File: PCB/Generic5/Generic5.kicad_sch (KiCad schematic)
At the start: 29 parts, among them J1 Conn_01x04, J2 USB-C, Q1 PMF170XP,115, U1 ESP32-PICO-MINI-02, U2 FT231XQ, U3 LMR16006+FB

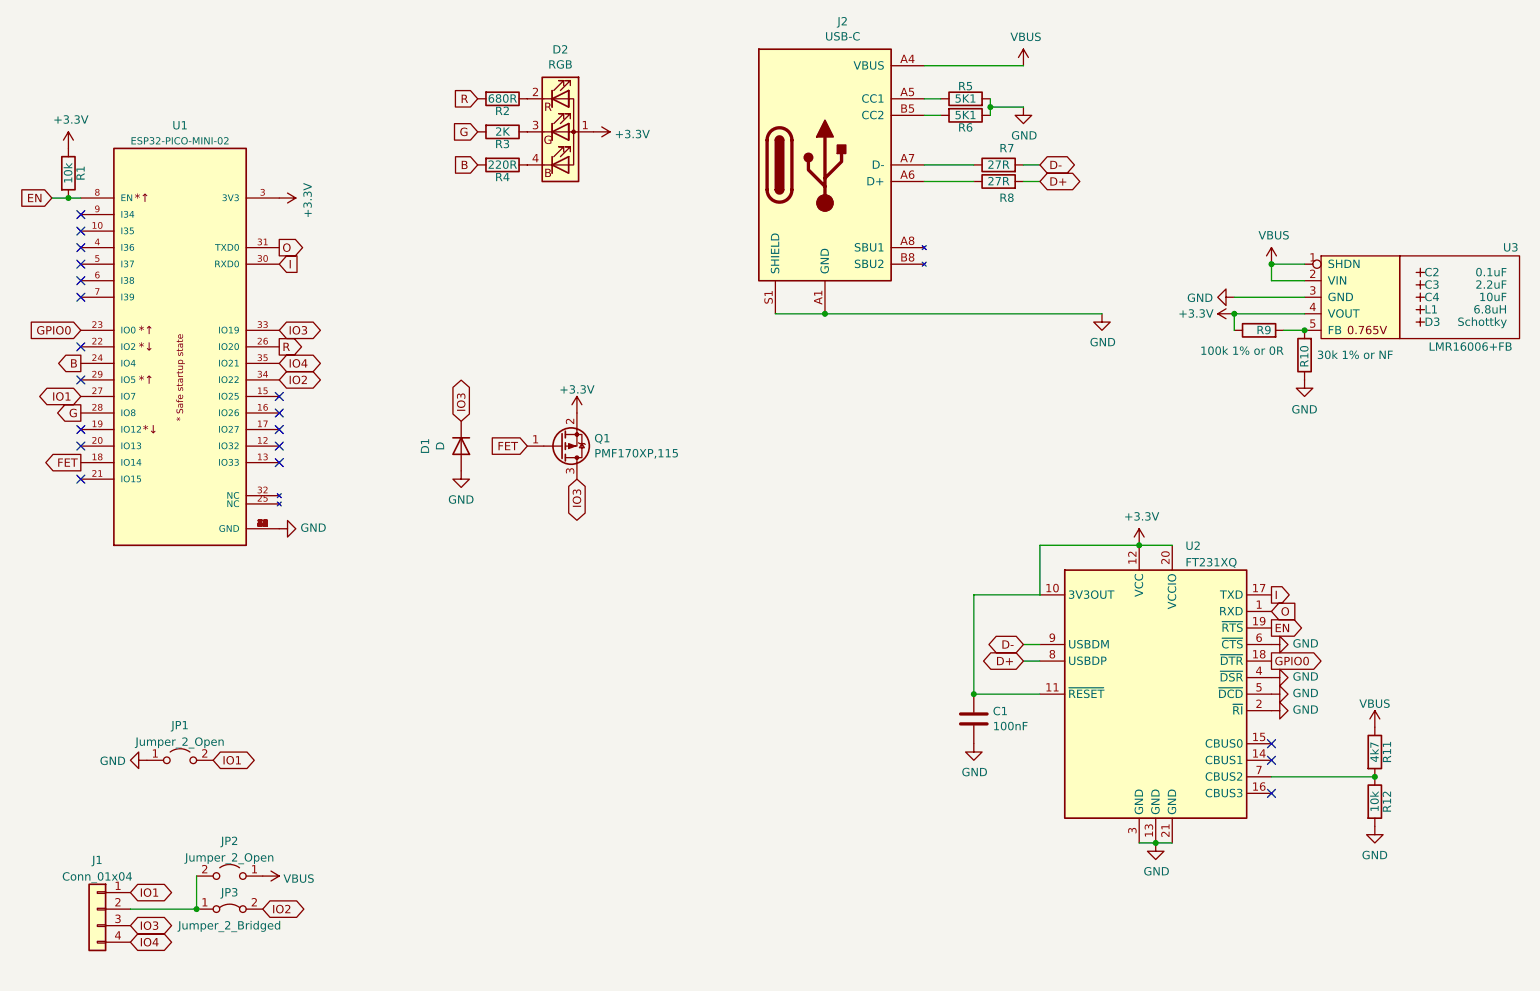
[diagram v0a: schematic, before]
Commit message: New LED Generic 5
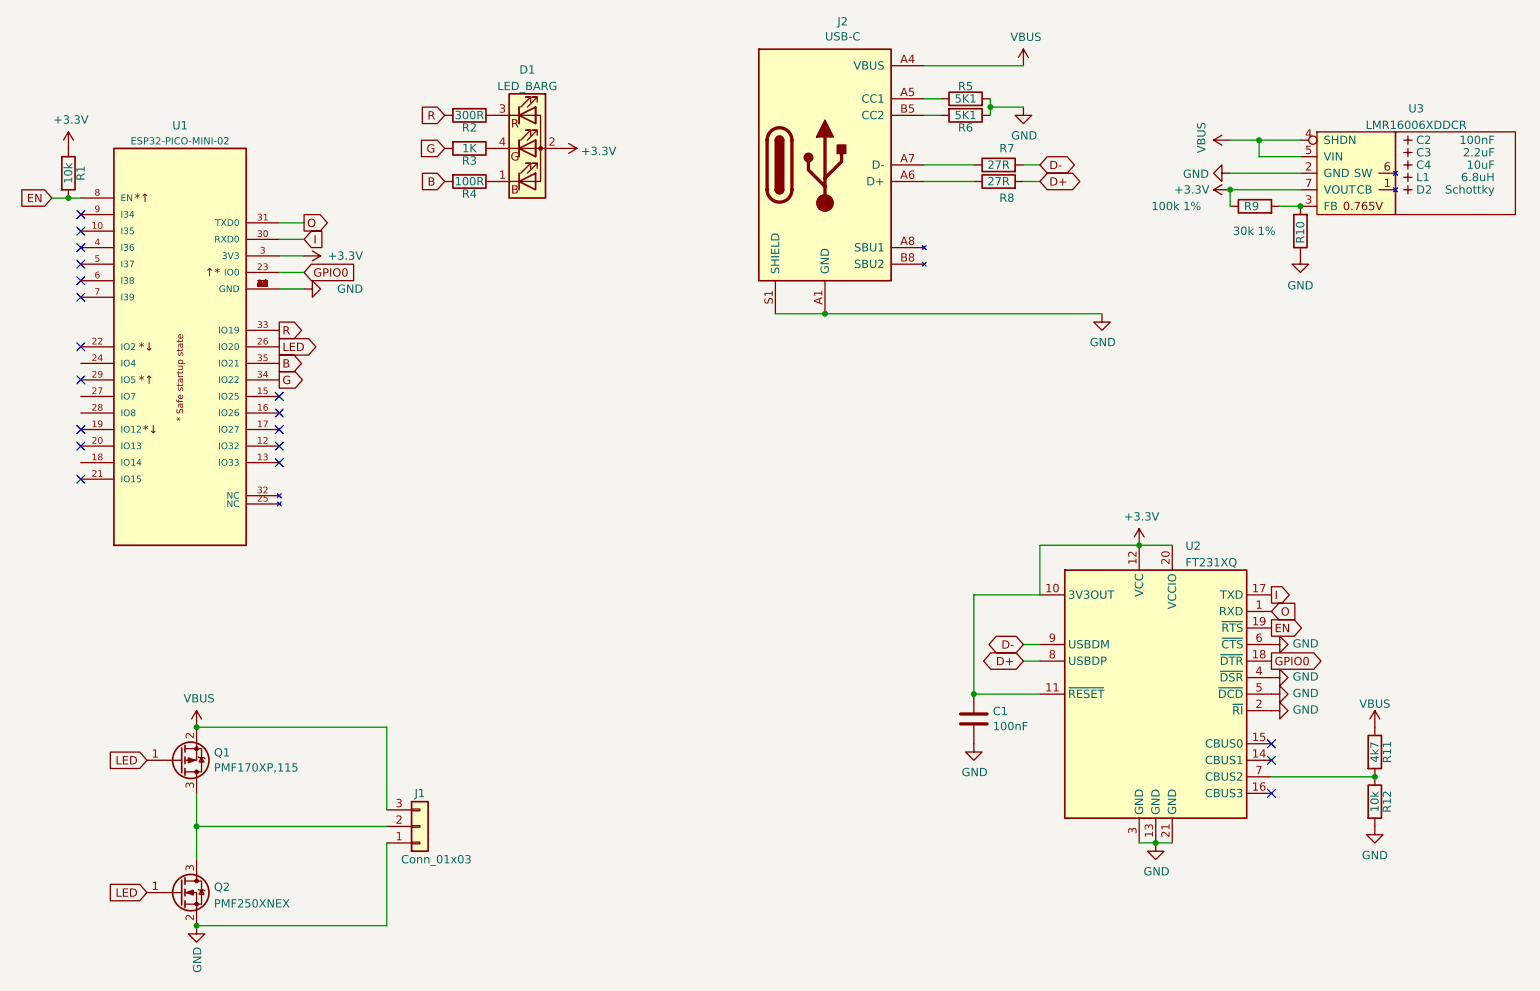
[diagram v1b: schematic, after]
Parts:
- removed D1: D, RevK:D_1206, symbol Device:D
- removed D2: RGB, RevK:LED-RGB-1.6x1.6, symbol Device:LED_ARGB
- removed D3: Schottky, RevK:Hidden, symbol RevK:Hidden
- removed J1: Conn_01x04, RevK:Molex_MiniSPOX_H4RA, symbol Connector_Generic:Conn_01x04
- removed JP1, JP2: Jumper_2_Open, RevK:Pad_0603_Open, symbol Jumper:Jumper_2_Open
- removed JP3: Jumper_2_Bridged, RevK:Pad_0603_Bridged, symbol Jumper:Jumper_2_Bridged
- removed U3: LMR16006+FB, RevK:RegulatorBlockFB, symbol RevK:LMR16006+FB
- added D1: LED_BARG, RevK:MHS190RGBCT, symbol Device:LED_BARG
- added D2: Schottky, RevK:D_1206_, symbol RevK:Hidden
- added J1: Conn_01x03, RevK:PTSM-HH-3-RA, symbol Connector_Generic:Conn_01x03
- added Q2: PMF250XNEX, RevK:SOT-323_SC-70, symbol RevK:NX7002AK
- added U3: LMR16006XDDCR, RevK:SOT-23-Thin-6-Reg, symbol RevK:LMR16006XDDCR
- C2: value 0.1uF -> 100nF; footprint RevK:Hidden -> RevK:C_0603_; LCSC Part # (none) -> C30926
- C3: footprint RevK:Hidden -> RevK:C_0805_; LCSC Part # (none) -> C19110; Note 0603 or 0805 -> (none)
- C4: footprint RevK:Hidden -> RevK:C_0805_; LCSC Part # (none) -> C17024; Note 0603 or 0805 -> (none)
- J2: footprint RevK:USC16-TR-Round -> RevK:USC16-TR-PTH
- L1: footprint RevK:Hidden -> RevK:L_4x4_; LCSC Part # (none) -> C354575; Manufacturer Laird -> (none); Part No TYA4020 -> (none)
- Q1: footprint Package_TO_SOT_SMD:SOT-323_SC-70 -> RevK:SOT-323_SC-70
- R10: value 30k 1% or NF -> 30k 1%; LCSC Part # (none) -> C100001
- R2: value 680R -> 300R; Part No (none) -> 0603-680R
- R3: value 2K -> 1K; Part No (none) -> 0603-2K
- R4: value 220R -> 100R; Part No (none) -> 0603-220R
- R9: value 100k 1% or 0R -> 100k 1%; LCSC Part # (none) -> C14675
- U1: LCSC Part # (none) -> C2980306
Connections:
- net IO2 is gone; now on net G: U1.34 (IO22)
- net IO4 is gone; now on net B: U1.35 (IO21)
- net +3V3: now also D1.2 (A), U3.7 (VOUT); no longer Q1.2 (S)
- net B: no longer U1.24 (IO4)
- net G: no longer U1.28 (IO8)
- net GND: now also J1.1 (Pin_1), Q2.2 (S), U3.2 (GND)
- net R: now also U1.33 (IO19); no longer U1.26 (IO20)
- net VBUS: now also Q1.2 (S), J1.3 (Pin_3), U3.4 (SHDN), U3.5 (VIN)
- net at R4.1: now also D1.1 (BK)
- net at R2.1: now also D1.3 (RK)
- net at R3.1: now also D1.4 (GK)
- net at R10.2, R9.2: now also U3.3 (FB)
- net FET: no longer names the net of U1.18 (IO14)
- net FET: no longer Q1.1 (G)
- net IO1: no longer names the net of U1.27 (IO7)
- net IO3: no longer names the net of Q1.3 (D)
- net IO3: now also J1.2 (Pin_2), Q2.3 (D); no longer U1.33 (IO19)
- new net LED: Q1.1 (G), Q2.1 (G), U1.26 (IO20)
